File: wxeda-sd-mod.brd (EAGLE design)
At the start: 101.3 x 40.6 mm, 23 parts, among them U1 SD_CARD, X2 TAPE IN / OUT

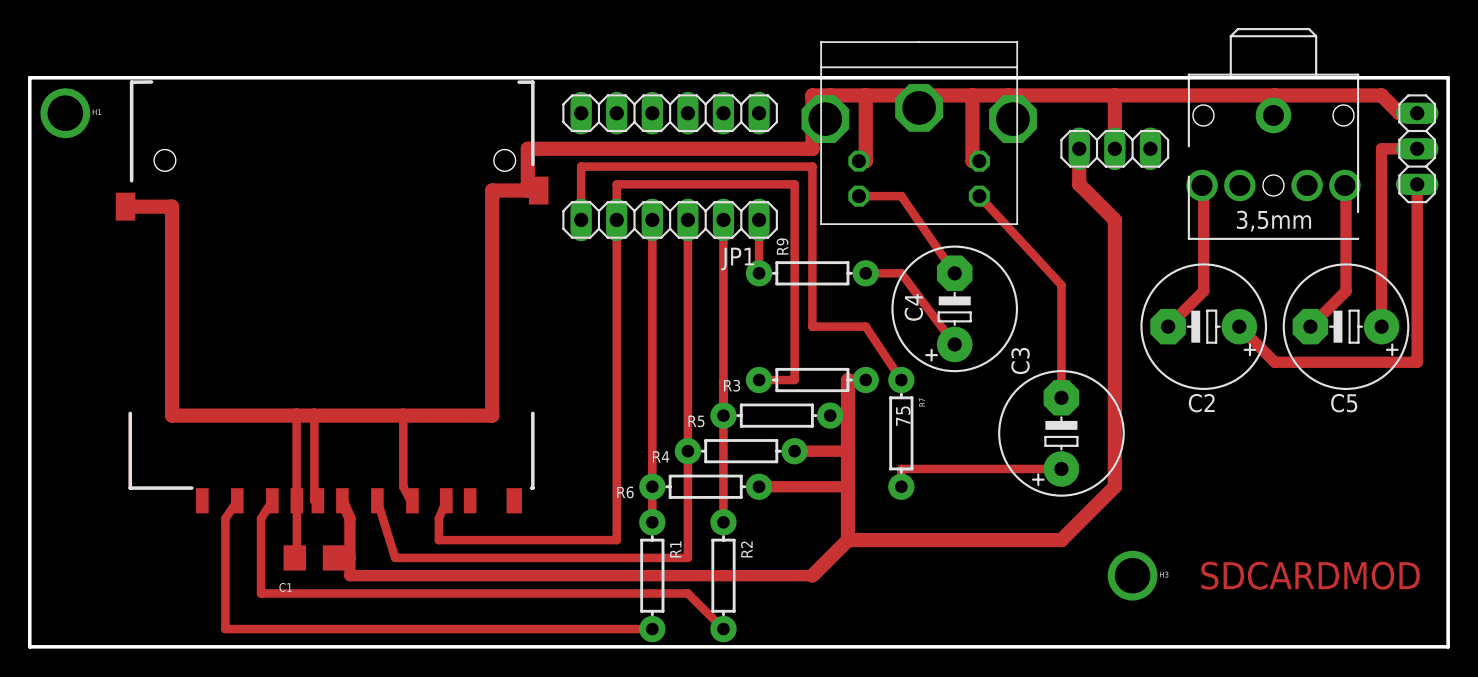
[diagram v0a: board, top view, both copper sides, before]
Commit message: release
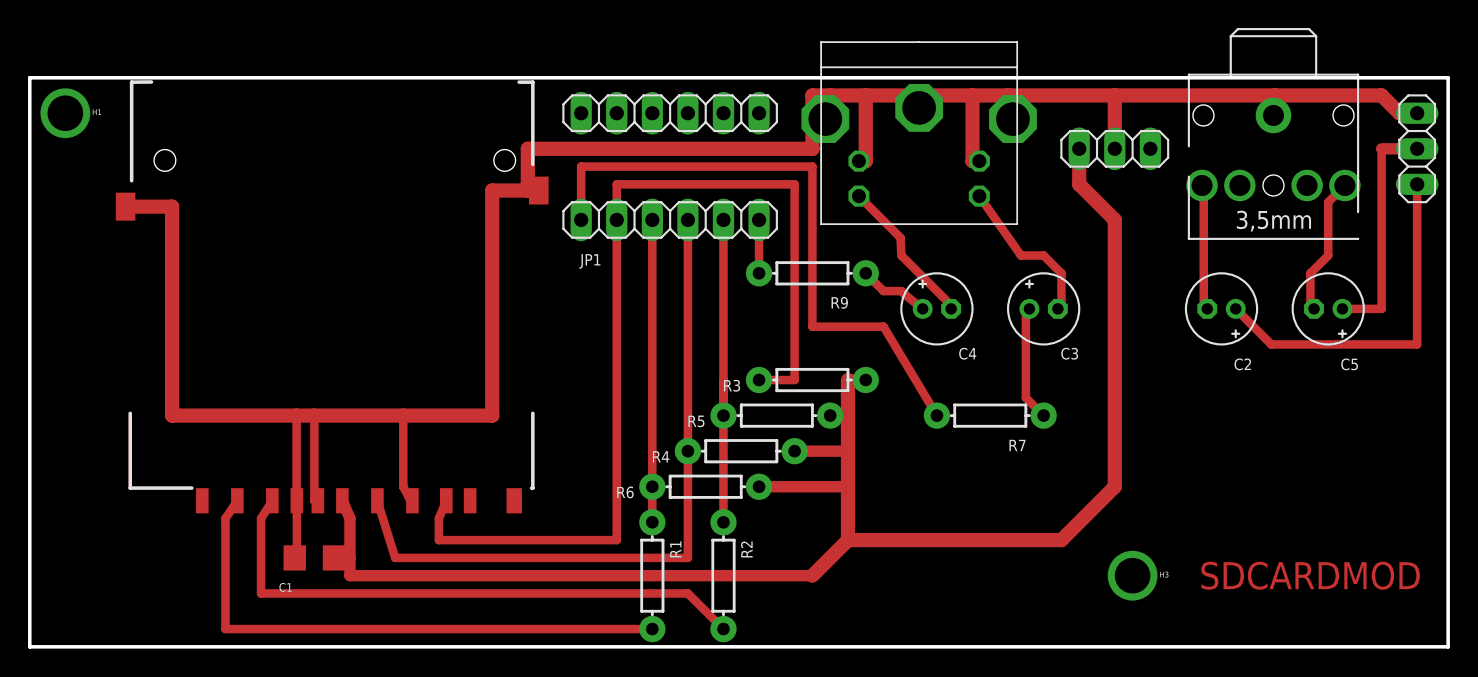
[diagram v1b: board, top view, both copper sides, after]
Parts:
- C2, C3, C4, C5: device adafruit:E5-8,5 -> adafruit:E2-5
- moved C3 8.98 mm to (72.4, 24.1), turned to 0 degrees
- moved R7 6.48 mm to (68.6, 16.5), turned to 0 degrees
- moved C2 1.80 mm to (85.1, 24.1)
- moved C5 1.80 mm to (92.7, 24.1)
- moved C4 1.27 mm to (64.8, 24.1), turned to 0 degrees
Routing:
- net Y_OUT: track 16.7 -> 11.4 mm
- net N$8: track 12.7 -> 8.25 mm
- net DSE: track 40.1 -> 44.2 mm
- net N$7: track 8.89 -> 5.05 mm
- net N$4: track 11.3 -> 9.23 mm
- net A_IN: track 15.2 -> 16.8 mm
- net C_OUT: track 9.73 -> 11.1 mm
- net N$6: track 11.2 -> 10.2 mm
- net GREEN: track 26.5 -> 25.4 mm
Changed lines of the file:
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@@
 <elements>
 <element name="JP1" library="pinhead" package="1X06" value="7SEG_LR" x="45.72" y="30.48" smashed="yes">
-<attribute name="NAME" x="49.4538" y="27.2288" size="1.27" layer="25" ratio="10"/>
+<attribute name="NAME" x="39.2938" y="27.2288" size="0.8128" layer="25" ratio="10"/>
 </element>
 <element name="JP2" library="pinhead" package="1X03" value="IRDA" x="77.47" y="35.56" smashed="yes" rot="R180"/>
 <element name="U1" library="SparkFun-Connectors" package="SDCARD_4UCONN" value="SD_CARD" x="21.59" y="11.43" smashed="yes" rot="R90">
-<attribute name="VALUE" x="17.54" y="22.13" size="1.27" layer="27" ratio="10"/>
+<attribute name="VALUE" x="8.65" y="13.24" size="0.8128" layer="27" ratio="10"/>
 </element>
 <element name="JP3" library="pinhead" package="1X06" value="7SEG_HR" x="45.72" y="38.1" smashed="yes"/>
@@
 <attribute name="NAME" x="43.18" y="11.43" size="0.8128" layer="25" font="vector" rot="R180"/>
 </element>
-<element name="C2" library="adafruit" package="E5-8,5" value="10uF" x="83.82" y="22.86" smashed="yes" rot="R180">
-<attribute name="NAME" x="84.7598" y="18.034" size="1.27" layer="25" ratio="10" rot="R180"/>
-<attribute name="VALUE" x="86.3346" y="25.8826" size="1.27" layer="27" ratio="10" rot="R180"/>
+<element name="C2" library="adafruit" package="E2-5" value="10uF" x="85.09" y="24.13" smashed="yes" rot="R180">
+<attribute name="NAME" x="87.2998" y="20.574" size="0.8128" layer="25" ratio="10" rot="R180"/>
 </element>
 <element name="R9" library="SparkFun-Passives" package="AXIAL-0.3" value="75" x="55.88" y="26.67" smashed="yes">
-<attribute name="NAME" x="53.34" y="29.2354" size="0.8128" layer="25" rot="R270"/>
-</element>
-<element name="C4" library="adafruit" package="E5-8,5" value="47uF" x="66.04" y="24.13" smashed="yes" rot="R90">
-<attribute name="NAME" x="63.754" y="23.1902" size="1.27" layer="25" ratio="10" rot="R90"/>
-<attribute name="VALUE" x="69.0626" y="21.6154" size="1.27" layer="27" ratio="10" rot="R90"/>
-</element>
-<element name="X2" library="adafruit" package="STX3100" value="TAPE IN / OUT" x="88.9" y="40.64" smashed="yes" rot="R270">
-<attribute name="VALUE" x="82.45" y="27.86" size="1.27" layer="27" ratio="10"/>
-</element>
-<element name="C5" library="adafruit" package="E5-8,5" value="10uF" x="93.98" y="22.86" smashed="yes" rot="R180">
-<attribute name="NAME" x="94.9198" y="18.034" size="1.27" layer="25" ratio="10" rot="R180"/>
-<attribute name="VALUE" x="96.4946" y="25.8826" size="1.27" layer="27" ratio="10" rot="R180"/>
-</element>
-<element name="R7" library="SparkFun-Passives" package="AXIAL-0.3" value="75" x="62.23" y="15.24" rot="R270"/>
-<element name="C3" library="adafruit" package="E5-8,5" value="47uF" x="73.66" y="15.24" rot="R90"/>
+<attribute name="NAME" x="57.15" y="24.1554" size="0.8128" layer="25"/>
+</element>
+<element name="C4" library="adafruit" package="E2-5" value="47uF" x="64.77" y="24.13" smashed="yes">
+<attribute name="NAME" x="67.6402" y="21.336" size="0.8128" layer="25" rot="R180"/>
+</element>
+<element name="X2" library="adafruit" package="STX3100" value="TAPE IN / OUT" x="88.9" y="40.64" smashed="yes" rot="R270"/>
+<element name="C5" library="adafruit" package="E2-5" value="10uF" x="92.71" y="24.13" smashed="yes" rot="R180">
+<attribute name="NAME" x="94.9198" y="20.574" size="0.8128" layer="25" ratio="10" rot="R180"/>
+</element>
+<element name="R7" library="SparkFun-Passives" package="AXIAL-0.3" value="75" x="68.58" y="16.51" smashed="yes">
+<attribute name="NAME" x="69.85" y="13.97" size="0.8128" layer="25" font="vector"/>
+</element>
+<element name="C3" library="adafruit" package="E2-5" value="47uF" x="72.39" y="24.13" smashed="yes">
+<attribute name="NAME" x="74.93" y="21.336" size="0.8128" layer="25" ratio="10" rot="R180"/>
+</element>
 <element name="U$1" library="connectors-digital" package="MINIDIN_4_3GND" value="S-VIDEO" x="63.5" y="43.18">
 <attribute name="PACKAGE" value="SHIELDED" x="63.5" y="43.18" size="1.778" layer="27" display="off"/>
@@
 <wire x1="58.42" y1="7.62" x2="58.42" y2="11.43" width="1.016" layer="1"/>
 <wire x1="58.42" y1="11.43" x2="58.42" y2="13.97" width="1.016" layer="1"/>
-<wire x1="58.42" y1="13.97" x2="58.42" y2="15.24" width="0" layer="19" extent="1-16"/>
 <wire x1="58.42" y1="13.97" x2="58.42" y2="16.51" width="1.016" layer="1"/>
 <wire x1="58.42" y1="16.51" x2="58.42" y2="19.05" width="1.016" layer="1"/>
@@
 <wire x1="54.61" y1="13.97" x2="58.42" y2="13.97" width="0.8128" layer="1"/>
 <wire x1="52.07" y1="11.43" x2="58.42" y2="11.43" width="0.8128" layer="1"/>
-<wire x1="62.23" y1="15.24" x2="58.42" y2="15.24" width="0" layer="19" extent="1-16"/>
 <wire x1="74.93" y1="35.56" x2="74.93" y2="33.02" width="1.016" layer="1"/>
 <wire x1="74.93" y1="33.02" x2="77.47" y2="30.48" width="1.016" layer="1"/>
@@
 <contactref element="JP1" pad="1"/>
 <contactref element="R7" pad="P$1"/>
-<wire x1="62.23" y1="19.05" x2="59.69" y2="22.86" width="0.6096" layer="1"/>
-<wire x1="59.69" y1="22.86" x2="55.88" y2="22.86" width="0.6096" layer="1"/>
+<wire x1="64.77" y1="16.51" x2="60.96" y2="22.86" width="0.6096" layer="1"/>
+<wire x1="60.96" y1="22.86" x2="55.88" y2="22.86" width="0.6096" layer="1"/>
 <wire x1="55.88" y1="22.86" x2="55.88" y2="34.29" width="0.6096" layer="1"/>
 <wire x1="55.88" y1="34.29" x2="39.37" y2="34.29" width="0.6096" layer="1"/>
@@
 <contactref element="C5" pad="+"/>
 <wire x1="99.06" y1="35.56" x2="96.52" y2="35.56" width="0.8128" layer="1"/>
-<wire x1="96.52" y1="35.56" x2="96.52" y2="22.86" width="0.8128" layer="1"/>
+<wire x1="96.52" y1="35.56" x2="96.52" y2="24.13" width="0.6096" layer="1"/>
+<wire x1="96.52" y1="24.13" x2="93.726" y2="24.13" width="0.6096" layer="1"/>
 </signal>
 <signal name="GREEN">
 <contactref element="JP4" pad="3"/>
 <contactref element="C2" pad="+"/>
-<wire x1="86.36" y1="22.86" x2="88.9" y2="20.32" width="0.8128" layer="1"/>
-<wire x1="88.9" y1="20.32" x2="99.06" y2="20.32" width="0.8128" layer="1"/>
-<wire x1="99.06" y1="20.32" x2="99.06" y2="33.02" width="0.8128" layer="1"/>
+<wire x1="86.106" y1="24.13" x2="88.646" y2="21.59" width="0.6096" layer="1"/>
+<wire x1="88.646" y1="21.59" x2="99.06" y2="21.59" width="0.6096" layer="1"/>
+<wire x1="99.06" y1="21.59" x2="99.06" y2="33.02" width="0.6096" layer="1"/>
 </signal>
 <signal name="N$1">
@@
 <contactref element="C2" pad="-"/>
 <wire x1="83.7" y1="32.94" x2="83.82" y2="32.94" width="0.6096" layer="1"/>
-<wire x1="83.82" y1="32.94" x2="83.82" y2="25.4" width="0.8128" layer="1"/>
-<wire x1="83.82" y1="25.4" x2="81.28" y2="22.86" width="0.8128" layer="1"/>
+<wire x1="83.7" y1="32.94" x2="83.82" y2="32.82" width="0.6096" layer="1"/>
+<wire x1="83.82" y1="32.82" x2="83.82" y2="24.13" width="0.6096" layer="1"/>
+<wire x1="83.82" y1="24.13" x2="84.074" y2="24.13" width="0.6096" layer="1"/>
 </signal>
 <signal name="N$6">
@@
 <contactref element="C5" pad="-"/>
 <wire x1="93.9" y1="32.94" x2="93.98" y2="32.94" width="0.8128" layer="1"/>
-<wire x1="93.98" y1="32.94" x2="93.98" y2="25.4" width="0.8128" layer="1"/>
-<wire x1="93.98" y1="25.4" x2="91.44" y2="22.86" width="0.8128" layer="1"/>
+<wire x1="93.9" y1="32.94" x2="92.71" y2="31.75" width="0.6096" layer="1"/>
+<wire x1="92.71" y1="31.75" x2="92.71" y2="27.94" width="0.6096" layer="1"/>
+<wire x1="92.71" y1="27.94" x2="91.44" y2="26.67" width="0.6096" layer="1"/>
+<wire x1="91.44" y1="26.67" x2="91.44" y2="24.13" width="0.6096" layer="1"/>
+<wire x1="91.44" y1="24.13" x2="91.694" y2="24.13" width="0.6096" layer="1"/>
 </signal>
 <signal name="N$7">
 <contactref element="R9" pad="P$2"/>
 <contactref element="C4" pad="+"/>
-<wire x1="59.69" y1="26.67" x2="62.23" y2="26.67" width="0.6096" layer="1"/>
-<wire x1="62.23" y1="26.67" x2="66.04" y2="21.59" width="0.6096" layer="1"/>
+<wire x1="59.69" y1="26.67" x2="60.96" y2="25.4" width="0.6096" layer="1"/>
+<wire x1="60.96" y1="25.4" x2="62.23" y2="25.4" width="0.6096" layer="1"/>
+<wire x1="62.23" y1="25.4" x2="62.484" y2="25.146" width="0.6096" layer="1"/>
+<wire x1="62.484" y1="25.146" x2="63.754" y2="24.13" width="0.6096" layer="1"/>
 </signal>
 <signal name="Y_OUT">
 <contactref element="U$1" pad="3"/>
 <contactref element="C3" pad="-"/>
-<wire x1="67.8" y1="32.18" x2="73.66" y2="25.83" width="0.6096" layer="1"/>
-<wire x1="73.66" y1="25.83" x2="73.66" y2="17.78" width="0.6096" layer="1"/>
+<wire x1="67.8" y1="32.18" x2="70.77" y2="27.94" width="0.6096" layer="1"/>
+<wire x1="70.77" y1="27.94" x2="72.39" y2="27.94" width="0.6096" layer="1"/>
+<wire x1="72.39" y1="27.94" x2="73.66" y2="26.67" width="0.6096" layer="1"/>
+<wire x1="73.66" y1="26.67" x2="73.66" y2="24.13" width="0.6096" layer="1"/>
+<wire x1="73.66" y1="24.13" x2="73.406" y2="24.13" width="0.6096" layer="1"/>
 </signal>
 <signal name="N$8">
 <contactref element="R7" pad="P$2"/>
 <contactref element="C3" pad="+"/>
-<wire x1="73.66" y1="12.7" x2="62.23" y2="12.7" width="0.6096" layer="1"/>
-<wire x1="62.23" y1="12.7" x2="62.23" y2="11.43" width="0.6096" layer="1"/>
+<wire x1="71.374" y1="24.13" x2="71.12" y2="23.876" width="0.6096" layer="1"/>
+<wire x1="71.12" y1="23.876" x2="71.12" y2="17.78" width="0.6096" layer="1"/>
+<wire x1="71.12" y1="17.78" x2="72.39" y2="16.51" width="0.6096" layer="1"/>
 </signal>
 <signal name="C_OUT">
 <contactref element="U$1" pad="4"/>
 <contactref element="C4" pad="-"/>
-<wire x1="59.2" y1="32.18" x2="62.23" y2="32.18" width="0.6096" layer="1"/>
-<wire x1="62.23" y1="32.18" x2="66.04" y2="26.67" width="0.6096" layer="1"/>
+<wire x1="59.2" y1="32.18" x2="62.17" y2="29.21" width="0.6096" layer="1"/>
+<wire x1="62.17" y1="29.21" x2="62.23" y2="27.94" width="0.6096" layer="1"/>
+<wire x1="62.23" y1="27.94" x2="66.04" y2="24.13" width="0.6096" layer="1"/>
+<wire x1="66.04" y1="24.13" x2="65.786" y2="24.13" width="0.6096" layer="1"/>
 </signal>
 </signals>
